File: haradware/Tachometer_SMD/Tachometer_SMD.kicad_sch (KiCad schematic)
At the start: 17 parts, among them J101 OUT_EX, J102 Battery, J103 ch2, J104 ch1, J105 Power_EX, SW101 SW_SPST, U101 LM393N

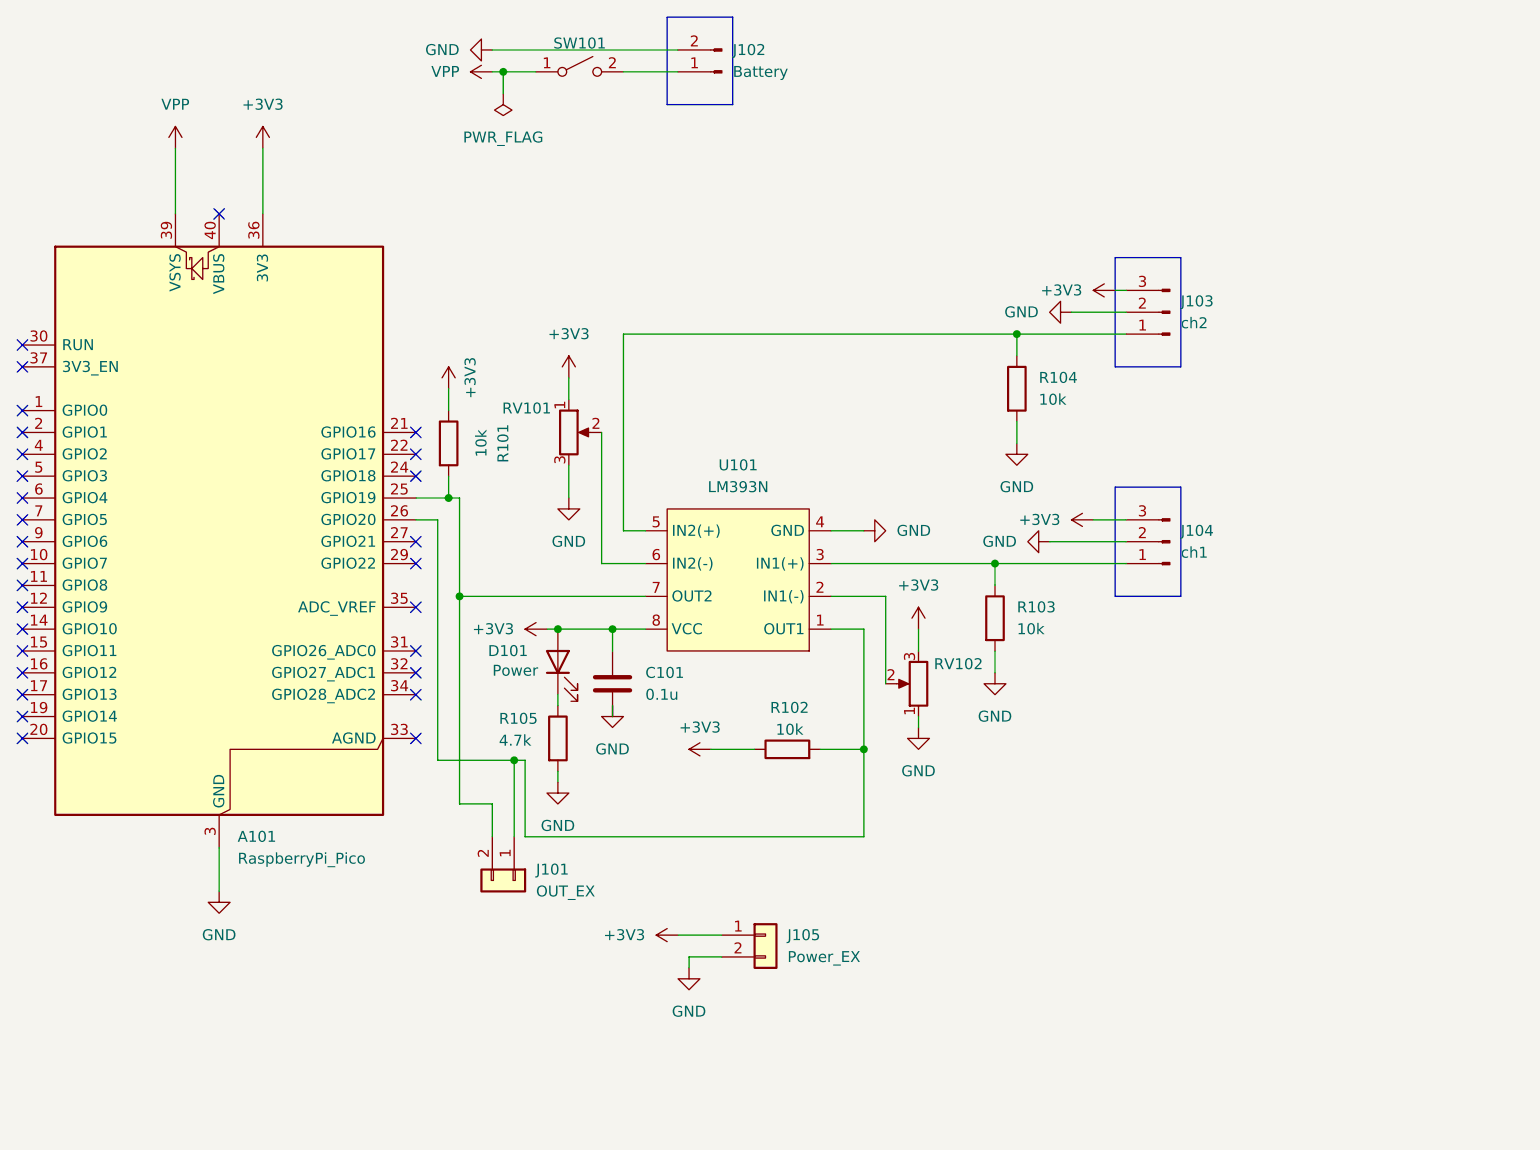
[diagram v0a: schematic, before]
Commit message: つくった
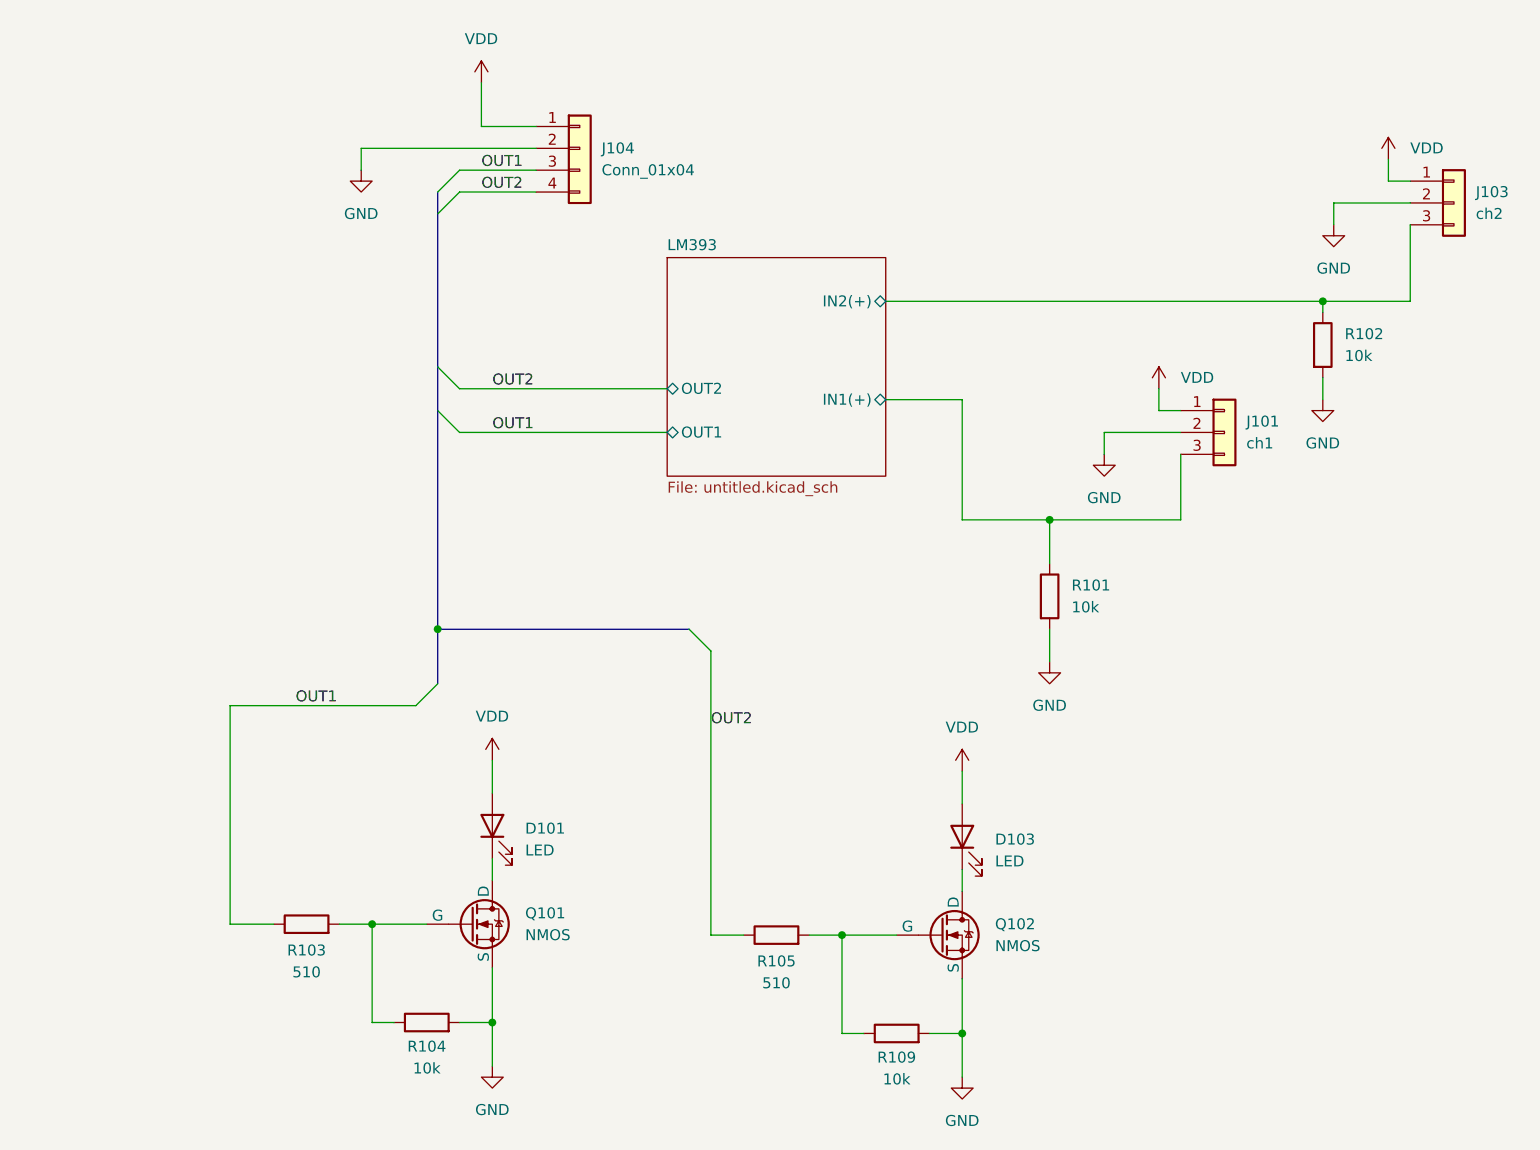
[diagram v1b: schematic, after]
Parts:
- removed A101: RaspberryPi_Pico, Module:RaspberryPi_Pico_Common_Unspecified, symbol MCU_Module:RaspberryPi_Pico
- removed C101: 0.1u, Capacitor_THT:C_Axial_L5.1mm_D3.1mm_P10.00mm_Horizontal, symbol Device:C
- removed J101: OUT_EX, Connector_PinHeader_2.54mm:PinHeader_1x02_P2.54mm_Vertical, symbol Connector_Generic:Conn_01x02
- removed J102: Battery, Connector_JST:JST_PH_B2B-PH-K_1x02_P2.00mm_Vertical, symbol Connector:Conn_01x02_Pin
- removed J103: ch2, Connector_JST:JST_PH_B3B-PH-K_1x03_P2.00mm_Vertical, symbol Connector:Conn_01x03_Pin
- removed J104: ch1, Connector_JST:JST_PH_B3B-PH-K_1x03_P2.00mm_Vertical, symbol Connector:Conn_01x03_Pin
- removed J105: Power_EX, Connector_PinHeader_2.54mm:PinHeader_1x02_P2.54mm_Vertical, symbol Connector_Generic:Conn_01x02
- removed RV101, RV102: R_Potentiometer, Potentiometer_THT:Potentiometer_Bourns_3296P_Horizontal, symbol Device:R_Potentiometer
- removed SW101: SW_SPST, Button_Switch_THT:SW_Slide-03_Wuerth-WS-SLTV_10x2.5x6.4_P2.54mm, symbol Switch:SW_SPST
- removed U101: LM393N, Package_DIP:CERDIP-8_W7.62mm_SideBrazed, symbol New_Library:LN393
- added D103: LED, symbol Device:LED
- added J101: ch1, symbol Connector_Generic:Conn_01x03
- added J103: ch2, symbol Connector_Generic:Conn_01x03
- added J104: Conn_01x04, symbol Connector_Generic:Conn_01x04
- added Q101, Q102: NMOS, symbol Simulation_SPICE:NMOS
- added R109: 10k, symbol Device:R
- D101: value Power -> LED; footprint LED_THT:LED_D5.0mm -> (none)
- R101, R102, R104: footprint Resistor_THT:R_Axial_DIN0207_L6.3mm_D2.5mm_P7.62mm_Horizontal -> (none)
- R103: value 10k -> 510; footprint Resistor_THT:R_Axial_DIN0207_L6.3mm_D2.5mm_P7.62mm_Horizontal -> (none)
- R105: value 4.7k -> 510; footprint Resistor_THT:R_Axial_DIN0207_L6.3mm_D2.5mm_P7.62mm_Horizontal -> (none)
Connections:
- net GND: now also R101.2, R102.2, J101.2 (Pin_2), J103.2 (Pin_2), J104.2 (Pin_2), Q101.3 (S), Q102.3 (S), R109.2; no longer R103.2, R105.2
- net at D101.1 (K): now also Q101.1 (D); no longer R105.1
- net OUT1: now reaches R103.1
- net OUT1: now also J104.3 (Pin_3)
- net at R104.1: now also R103.2, Q101.2 (G)
- removed net +3V3: D101.2 (A), R101.1, R102.1
- new net: D103.1 (K), Q102.1 (D)
- new net: Q102.2 (G), R105.2, R109.1
- new net LM393/IN1(+): J101.3 (Pin_3), R101.1
- new net LM393/IN2(+): J103.3 (Pin_3), R102.1
- new net OUT2: J104.4 (Pin_4), R105.1
- new net VDD: D101.2 (A), D103.2 (A), J101.1 (Pin_1), J103.1 (Pin_1), J104.1 (Pin_1)
- no-connect marks 29 -> 0
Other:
- added sheet LM393 (untitled.kicad_sch)
